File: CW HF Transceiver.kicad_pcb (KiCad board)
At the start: 2 copper layers, 42 parts, among them U4 Si5351A-B-GT, U5 MCP1700x-500xxMB

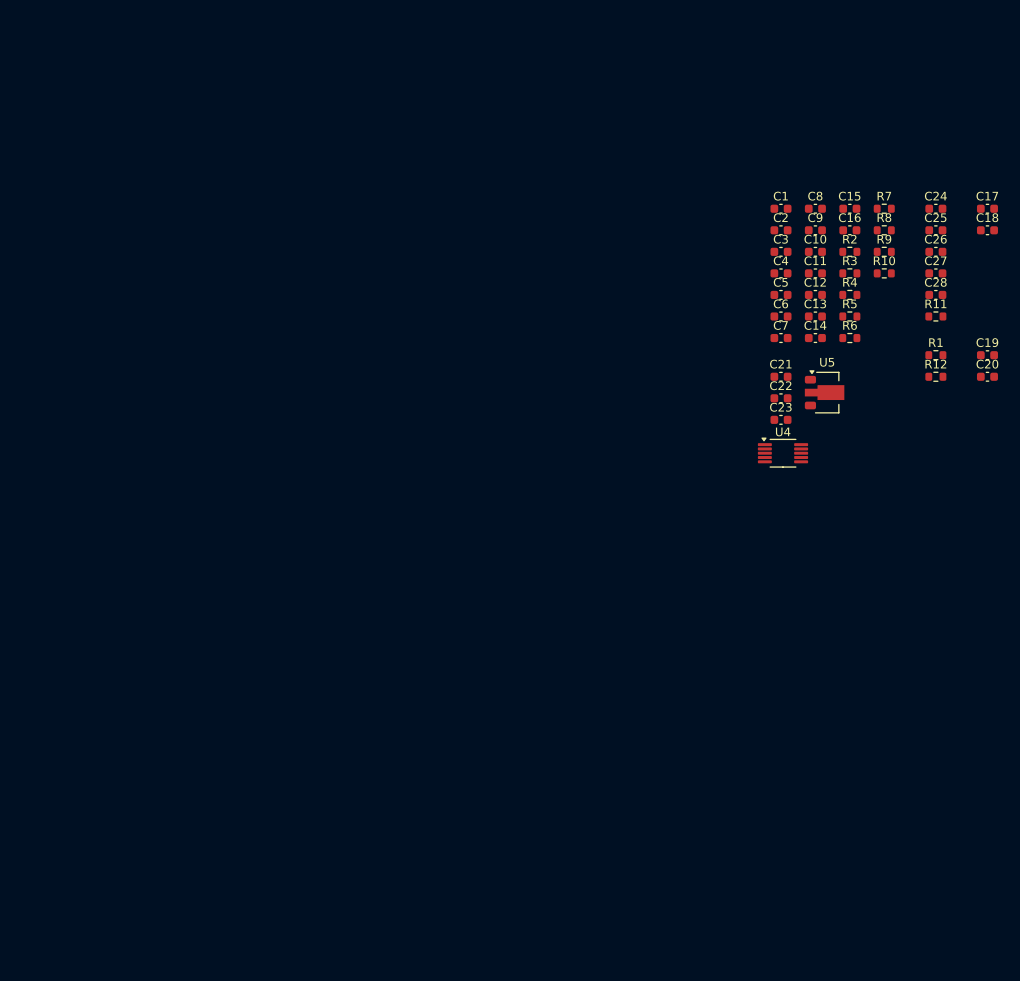
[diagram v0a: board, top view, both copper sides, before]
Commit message: add the pcb
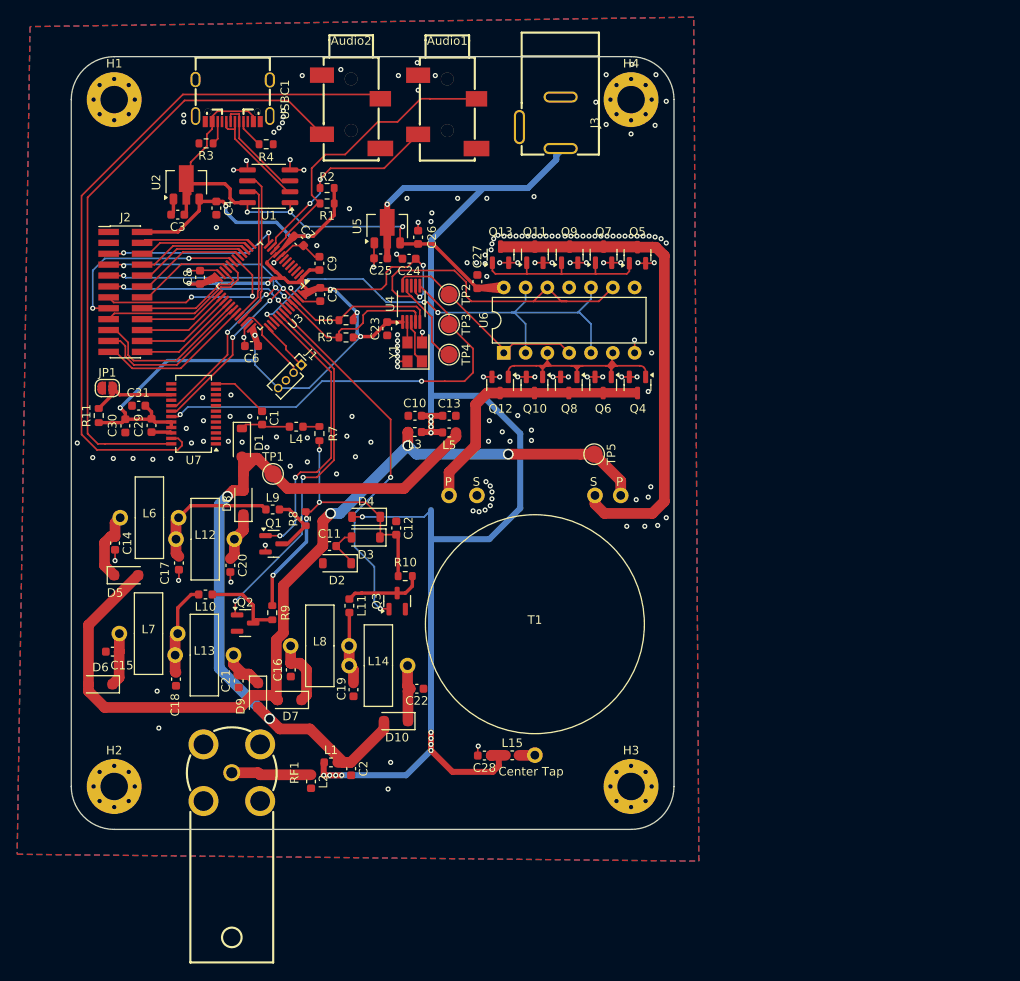
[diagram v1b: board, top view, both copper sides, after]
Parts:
- removed R12: 4.7k, Resistor_SMD:R_0603_1608Metric
- added Audio1: PJ-327C-4A, plib:AUDIO-SMD_PJ-327C-4A, F.Cu at (157.8, 53.7)
- added Audio2: PJ-327C-4A, plib:AUDIO-SMD_PJ-327C-4A, F.Cu at (146.6, 53.7)
- added C29: 22n, Capacitor_SMD:C_0603_1608Metric, F.Cu at (123.3, 90.3)
- added C30: 100n, Capacitor_SMD:C_0603_1608Metric, F.Cu at (120.3, 90.3)
- added C31: 100n, Capacitor_SMD:C_0603_1608Metric, F.Cu at (121.8, 88.0)
- added D1: 1N4007, Diode_SMD:D_SOD-123, F.Cu at (133.9, 92.2)
- added D10: 1N4007, Diode_SMD:D_SOD-123F, F.Cu at (151.8, 124.7)
- added D2: 1N4148, Diode_SMD:D_SOD-123, F.Cu at (144.9, 106.3)
- added D3: 1N4148, Diode_SMD:D_SOD-123, F.Cu at (148.3, 103.3)
- added D4: 1N4148, Diode_SMD:D_SOD-123, F.Cu at (148.3, 100.9)
- added D5: 1N4007, Diode_SMD:D_SOD-123F, F.Cu at (120.4, 107.7)
- added D6: 1N4007, Diode_SMD:D_SOD-123F, F.Cu at (117.4, 120.4)
- added D7: 1N4007, Diode_SMD:D_SOD-123F, F.Cu at (139.4, 122.2)
- added D8: 1N4007, Diode_SMD:D_SOD-123F, F.Cu at (134.1, 99.2)
- added D9: 1N4007, Diode_SMD:D_SOD-123F, F.Cu at (135.8, 121.7)
- added H1: MountingHole_Pad, MountingHole:MountingHole_3.2mm_M3_Pad_Via, F.Cu at (119.0, 52.3)
- added H2: MountingHole_Pad, MountingHole:MountingHole_3.2mm_M3_Pad_Via, F.Cu at (119.0, 132.3)
- added H3: MountingHole_Pad, MountingHole:MountingHole_3.2mm_M3_Pad_Via, F.Cu at (179.2, 132.3)
- added H4: MountingHole_Pad, MountingHole:MountingHole_3.2mm_M3_Pad_Via, F.Cu at (179.2, 52.3)
- added J1: JTAG, Connector_PinHeader_1.27mm:PinHeader_1x04_P1.27mm_Vertical, F.Cu at (140.8, 83.2)
- added J2: Conn_02x12_Odd_Even, Connector_PinHeader_1.27mm:PinHeader_2x12_P1.27mm_Vertical_SMD, F.Cu at (120.3, 74.7)
- added J3: Barrel_Jack_Switch, plib:DC-IN-TH_DC-5520-1, F.Cu at (168.6, 55.0)
- added JP1: RST RX, Jumper:SolderJumper-2_P1.3mm_Open_RoundedPad1.0x1.5mm, F.Cu at (118.2, 85.9)
- added L1: L, Inductor_SMD:L_0603_1608Metric, F.Cu at (144.2, 129.5)
- added L10: L, Inductor_SMD:L_0603_1608Metric, F.Cu at (129.6, 109.9)
- added L11: L, Inductor_SMD:L_0603_1608Metric, F.Cu at (146.4, 111.3)
- added L12: 330n, plib:ft37-67, F.Cu at (129.6, 103.5)
- added L13: 560n, plib:ft37-67, F.Cu at (129.5, 117.0)
- added L14: 1.3u, plib:ft37-67, F.Cu at (149.8, 118.2)
- added L15: L, Inductor_SMD:L_0603_1608Metric, F.Cu at (165.4, 128.7)
- added L2: L, Inductor_SMD:L_0603_1608Metric, F.Cu at (141.9, 131.7)
- added L3: L, Inductor_SMD:L_0603_1608Metric, F.Cu at (154.0, 91.0)
- added L4: L, Inductor_SMD:L_0603_1608Metric, F.Cu at (140.2, 90.4)
- added L5: L, Inductor_SMD:L_0603_1608Metric, F.Cu at (158.0, 91.1)
- added L6: 330n, plib:ft37-67, F.Cu at (123.1, 101.0)
- added L7: 560n, plib:ft37-67, F.Cu at (123.0, 114.5)
- added L8: 1.5u, plib:ft37-67, F.Cu at (142.9, 115.9)
- added L9: L, Inductor_SMD:L_0603_1608Metric, F.Cu at (137.5, 100.0)
- added Q1: BSS123, Package_TO_SOT_SMD:SOT-23, F.Cu at (137.6, 104.0)
- added Q10: BSS123, Package_TO_SOT_SMD:SOT-23, F.Cu at (167.9, 85.5)
- added Q11: BSS123, Package_TO_SOT_SMD:SOT-23, F.Cu at (168.0, 70.4)
- added Q12: BSS123, Package_TO_SOT_SMD:SOT-23, F.Cu at (163.9, 85.5)
- added Q13: BSS123, Package_TO_SOT_SMD:SOT-23, F.Cu at (164.0, 70.4)
- added Q2: BSS123, Package_TO_SOT_SMD:SOT-23, F.Cu at (134.3, 113.3)
- added Q3: BSS123, Package_TO_SOT_SMD:SOT-23, F.Cu at (152.0, 110.7)
- added Q4: BSS123, Package_TO_SOT_SMD:SOT-23, F.Cu at (179.9, 85.5)
- added Q5: BSS123, Package_TO_SOT_SMD:SOT-23, F.Cu at (179.9, 70.4)
- added Q6: BSS123, Package_TO_SOT_SMD:SOT-23, F.Cu at (175.9, 85.5)
- added Q7: BSS123, Package_TO_SOT_SMD:SOT-23, F.Cu at (176.0, 70.4)
- added Q8: BSS123, Package_TO_SOT_SMD:SOT-23, F.Cu at (171.9, 85.5)
- added Q9: BSS123, Package_TO_SOT_SMD:SOT-23, F.Cu at (172.1, 70.4)
- added RF1: DOSIN-801-0050, plib:BNC-TH_DOSIN-801-0051, F.Cu at (132.7, 130.7)
- added T1: 1:2, plib:ft50-75 trafo with CT, F.Cu at (168.0, 113.4)
- added TP1: Filters out, TestPoint:TestPoint_Pad_D2.0mm, F.Cu at (137.5, 95.9)
- added TP2: CLK0, TestPoint:TestPoint_Pad_D2.0mm, F.Cu at (158.0, 75.0)
- added TP3: CLK2, TestPoint:TestPoint_Pad_D2.0mm, F.Cu at (158.0, 78.5)
- added TP4: CLK1, TestPoint:TestPoint_Pad_D2.0mm, F.Cu at (158.0, 82.0)
- added TP5: Amp Out, TestPoint:TestPoint_Pad_D2.0mm, F.Cu at (174.9, 93.6)
- added U1: USB6B1, Package_SO:SOIC-8_3.9x4.9mm_P1.27mm, F.Cu at (137.0, 62.4)
- added U2: MCP1700x-330xxMB, Package_TO_SOT_SMD:SOT-89-3, F.Cu at (127.4, 61.9)
- added U3: STM32F072C8Tx, Package_QFP:LQFP-48_7x7mm_P0.5mm, F.Cu at (136.0, 74.0)
- added U6: 74ACT08, Package_DIP:DIP-14_W7.62mm, F.Cu at (164.4, 81.8)
- added U7: Si4735-D60-GU, Package_SO:SSOP-24_3.9x8.7mm_P0.635mm, F.Cu at (128.2, 88.9)
- added USBC1: USB3.1C16PFSMT, plib:USB-C-SMD_TYPE-C-USB-17, F.Cu at (132.8, 52.4)
- added Y1: NX3225GA-25.000M-STD-CRG-2, Crystal:Crystal_SMD_3225-4Pin_3.2x2.5mm, F.Cu at (154.0, 81.7)
- C1, C2: value 22u -> C
- C10: value 1u -> C
- C11, C12, C13, C28: value 100n -> C
- C14: value 100n -> 110p
- C15: value 100n -> 180p
- C16: value 100n -> 470p
- C17: value 1p -> 180p
- C18: value 1p -> 300p
- C19: value 1u -> 750p
- C20: value 1u -> 91p
- C21: value 22u -> 160p
- C22: value 22u -> 430p
- C23: value 100n -> 1u
- C24: value 22p -> 1u
- C25: value 22p -> 22u
- C26: value 22n -> 22u
- C3: value 100n -> 22u
- C4: value 15p -> 22u
- C5: value 15p -> 100n
- C8: value 1u -> 100n
- R1: value R -> 4.7k
- R10, R8, R9: value 1k -> R
- R2: value 5k1 -> 4.7k
- R4: value 1k -> 5k1
- R5: value 10k -> 1k
- R6: value 27.4 -> 1k
- R7: value 27.4 -> R
- moved C18 108.0 mm to (126.2, 119.8), turned to -90 degrees
- moved C17 102.8 mm to (126.5, 106.3), turned to -90 degrees
- moved C15 100.2 mm to (118.8, 116.6), turned to 180 degrees
- moved R11 98.2 mm to (117.2, 89.1), turned to 90 degrees
- moved C20 90.9 mm to (132.5, 106.5), turned to -90 degrees
- moved C14 85.0 mm to (119.1, 104.0), turned to -90 degrees
- moved C19 83.5 mm to (146.9, 121.0), turned to -90 degrees
- moved C16 82.8 mm to (139.6, 118.7), turned to -90 degrees
- moved R9 82.8 mm to (137.4, 112.1), turned to 90 degrees
- moved C2 80.2 mm to (146.6, 130.2), turned to -90 degrees
- moved R3 76.5 mm to (129.7, 57.4), turned to 180 degrees
- moved R8 75.3 mm to (141.3, 101.1), turned to 90 degrees
- moved C28 75.1 mm to (162.1, 128.7), turned to 180 degrees
- moved R1 73.1 mm to (143.8, 64.4), turned to 180 degrees
- moved C21 72.4 mm to (133.5, 120.0), turned to -90 degrees
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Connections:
- C1 pad 1: +5V -> /Receiver/Input
- C1 pad 2: GND -> /Filtering/t/r rbias
- C10 pad 1: +3.3V -> VCC
- C11 pad 1: +3.3V -> /Filtering/Input Bias
- C11 pad 2: Net-(C11-Pad2) -> Net-(D2-K)
- C12 pad 1: +3.3V -> GND
- C12 pad 2: Net-(C11-Pad2) -> /Filtering/voltage tripler
- C13 pad 1: +3.3V -> VCC
- C13 pad 2: Net-(C11-Pad2) -> GND
- C14 pad 1: +3.3V -> Net-(D5-K)
- C14 pad 2: Net-(C11-Pad2) -> GND
- C15 pad 1: +3.3V -> Net-(D6-K)
- C15 pad 2: Net-(C11-Pad2) -> GND
- C16 pad 1: +3.3V -> Net-(D7-K)
- C16 pad 2: Net-(C11-Pad2) -> GND
- C19 pad 1: +3.3V -> Net-(C19-Pad1)
- C2 pad 1: +3.3V -> /Filtering/Output Bias
- C2 pad 2: GND -> /ant
- C20 pad 1: VCC -> Net-(D8-K)
- C21 pad 1: Vdrive -> Net-(D9-K)
- C22 pad 1: +5V -> Net-(D10-K)
- C23 pad 1: +5V -> +3.3V
- C24 pad 1: /Receiver/DCLK -> +3.3V
- C25 pad 1: /Receiver/RCLK -> VCC
- C26 pad 1: +3.3V -> +5V
- C26 pad 2: Net-(U7-DBYP) -> GND
- C27 pad 1: +3.3V -> +5V
- C28 pad 1: +3.3V -> VCC
- C3 pad 1: +3.3V -> +5V
- C4 pad 1: GND -> +3.3V
- C4 pad 2: Net-(U3-XIN) -> GND
- C5 pad 1: GND -> +3.3V
- C5 pad 2: Net-(C5-Pad2) -> GND
- C6 pad 1: +1V1 -> +3.3V
- C7 pad 1: +1V1 -> +3.3V
- C8 pad 1: +1V1 -> +3.3V
- C9 pad 2: Net-(C11-Pad2) -> GND
- R1 pad 1: VCC -> +3.3V
- R1 pad 2: Vdrive -> /dit
- R10 pad 1: +3.3V -> Net-(Q3-D)
- R10 pad 2: /RP2040 Driver/sda -> /Filtering/voltage tripler
- R2 pad 1: Net-(J6-CC2) -> +3.3V
- R2 pad 2: GND -> /dah
- R4 pad 2: /RP2040 Driver/QSPI_SS -> GND
- R5 pad 2: /RP2040 Driver/QSPI_SS -> /STM32 Driver/scl
- R6 pad 1: /RP2040 Driver/D+ -> +3.3V
- R6 pad 2: Net-(U3-USB_DP) -> /STM32 Driver/sda
- R7 pad 1: /RP2040 Driver/D- -> /Filtering/voltage tripler
- R8 pad 1: Net-(C5-Pad2) -> Net-(Q1-D)
- R8 pad 2: Net-(U3-XOUT) -> /Filtering/voltage tripler
- R9 pad 1: +3.3V -> Net-(Q2-D)
- R9 pad 2: /RP2040 Driver/scl -> /Filtering/voltage tripler
- U4 pad 4: /RP2040 Driver/scl -> /STM32 Driver/scl
- U4 pad 5: /RP2040 Driver/sda -> /STM32 Driver/sda
- U4 pad 6: /Square Wave Gen/BFO out -> /Receiver/Receiver clk
- U5 pad 2: Vdrive -> VCC
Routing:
- net VCC: track 0.00 -> 169.4 mm, vias 0 -> 14
- net +3.3V: track 0.00 -> 141.6 mm, vias 0 -> 11
- net /Filtering/Input Bias: track 0.00 -> 106.0 mm, vias 0 -> 3
- net /Filtering/Output Bias: track 0.00 -> 86.8 mm, vias 0 -> 2
- net /Receiver/Rout: track 0.00 -> 82.2 mm
- net /Receiver/Lout: track 0.00 -> 71.4 mm
- net +5V: track 0.00 -> 63.2 mm, vias 0 -> 3
- net /STM32 Driver/scl: track 0.00 -> 62.3 mm, vias 0 -> 5
- net /STM32 Driver/sda: track 0.00 -> 61.6 mm, vias 0 -> 4
- net /Amplifier/Amp enable: track 0.00 -> 58.8 mm, vias 0 -> 3
- net GND: track 0.00 -> 58.7 mm, vias 0 -> 166
- net /Receiver/Receiver clk: track 0.00 -> 50.0 mm, vias 0 -> 2
- net /Amplifier/180º Wave: track 0.00 -> 48.9 mm
- net /Filtering/Filter 3 En: track 0.00 -> 43.6 mm, vias 0 -> 2
- net /Filtering/Filter 2 En: track 0.00 -> 43.2 mm, vias 0 -> 2
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- added copper zone on B.Cu, net GND
- added copper zone on F.Cu, net GND
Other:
- board outline added: 70.2 x 90 mm
- board text added: "S"
